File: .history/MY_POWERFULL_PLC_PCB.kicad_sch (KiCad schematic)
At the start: 6 parts, among them J1 DI_IN_Connector, J2 DI_IN_Connector, J3 DI_IN_Connector, J4 DI_IN_Connector, J5 DI_IN_Connector, J6 DI_IN_Connector

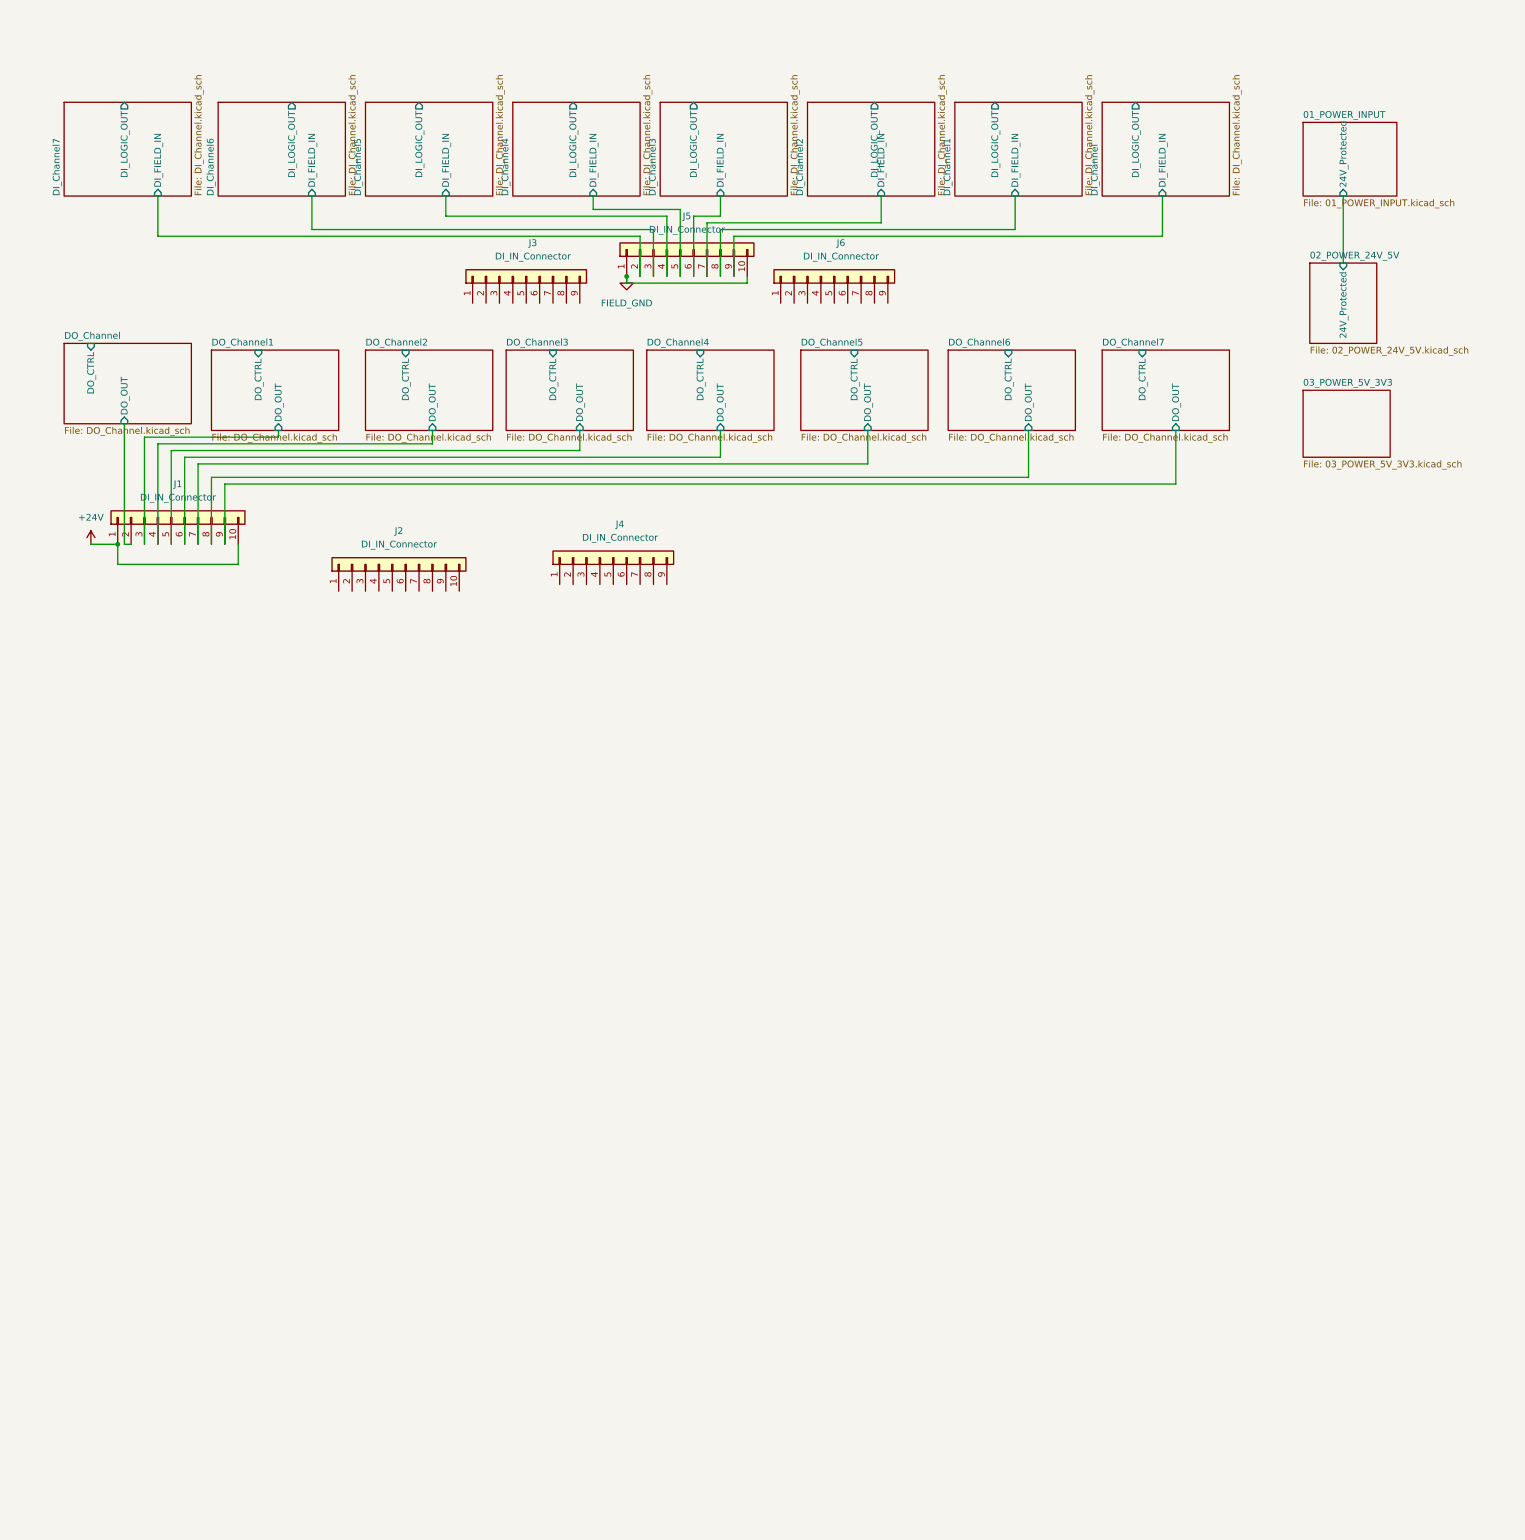
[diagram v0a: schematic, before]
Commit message: 112
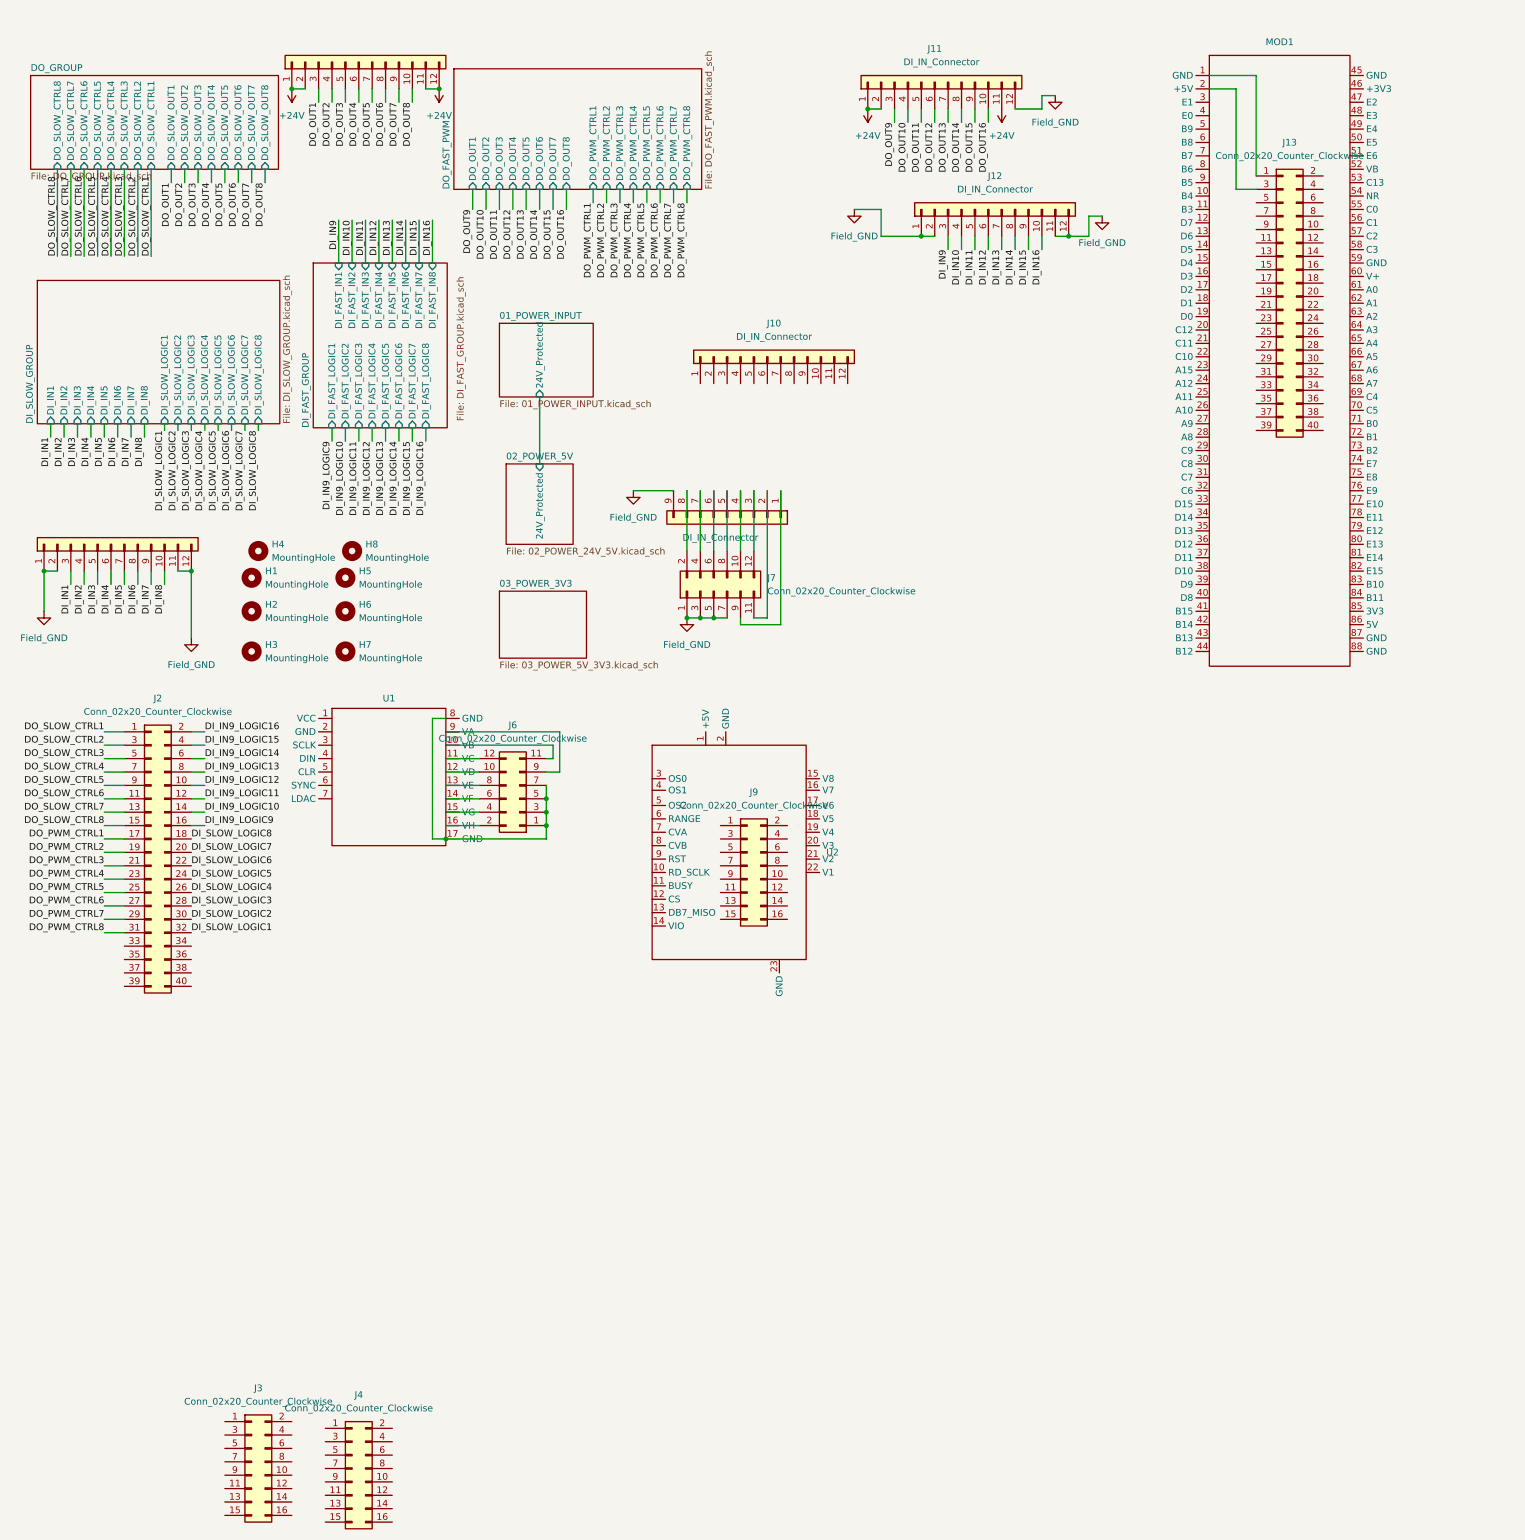
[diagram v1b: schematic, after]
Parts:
- removed J4: DI_IN_Connector, Connector_Phoenix_MC:PhoenixContact_MC_1,5_10-G-3.81_1x10_P3.81mm_Horizontal, symbol Connector_Generic:Conn_01x09
- added H1, H2, H3, H4, H5, H6, H7, H8: MountingHole, MountingHole:MountingHole_3.2mm_M3_Pad, symbol Mechanical:MountingHole
- added J13, J2: Conn_02x20_Counter_Clockwise, Connector_IDC:IDC-Header_2x20_P2.54mm_Vertical, symbol Connector_Generic:Conn_02x20_Odd_Even
- added J3, J4, J9: Conn_02x20_Counter_Clockwise, Connector_IDC:IDC-Header_2x08_P2.54mm_Vertical, symbol Connector_Generic:Conn_02x08_Odd_Even
- added J6, J7: Conn_02x20_Counter_Clockwise, Connector_IDC:IDC-Header_2x06_P2.54mm_Vertical, symbol Connector_Generic:Conn_02x06_Odd_Even
- added J8: DI_IN_Connector, Connector_Phoenix_MC:PhoenixContact_MC_1,5_9-G-3.5_1x09_P3.50mm_Horizontal, symbol Connector_Generic:Conn_01x09
- added MOD1: (no value), MyModules:WeAct_STM32H743VIT6, symbol MyModules:WeAct_STM32H743VIT6
- added U1: (no value), MyModules:DAC8568_Module_57x52mm, symbol MyModules:Module_DAC8568_8CH
- added U2: (no value), MyModules:AD7606_Module_40x30mm, symbol MyModules:Module_AD7606_8CH
- J1: renamed from J5; footprint Connector_Phoenix_MC:PhoenixContact_MC_1,5_10-G-3.81_1x10_P3.81mm_Horizontal -> Connector_Phoenix_MC:PhoenixContact_MC_1,5_12-G-3.5_1x12_P3.50mm_Horizontal; symbol Connector_Generic:Conn_01x10 -> Connector_Generic:Conn_01x12
- J10: renamed from J3; footprint Connector_Phoenix_MC:PhoenixContact_MC_1,5_10-G-3.81_1x10_P3.81mm_Horizontal -> Connector_Phoenix_MC:PhoenixContact_MC_1,5_12-G-3.5_1x12_P3.50mm_Horizontal; symbol Connector_Generic:Conn_01x09 -> Connector_Generic:Conn_01x12
- J11: renamed from J6; footprint Connector_Phoenix_MC:PhoenixContact_MC_1,5_10-G-3.81_1x10_P3.81mm_Horizontal -> Connector_Phoenix_MC:PhoenixContact_MC_1,5_12-G-3.5_1x12_P3.50mm_Horizontal; symbol Connector_Generic:Conn_01x09 -> Connector_Generic:Conn_01x12
- J12: renamed from J2; footprint Connector_Phoenix_MC:PhoenixContact_MC_1,5_10-G-3.81_1x10_P3.81mm_Horizontal -> Connector_Phoenix_MC:PhoenixContact_MC_1,5_12-G-3.5_1x12_P3.50mm_Horizontal; symbol Connector_Generic:Conn_01x10 -> Connector_Generic:Conn_01x12
- J5: renamed from J1; footprint Connector_Phoenix_MC:PhoenixContact_MC_1,5_10-G-3.81_1x10_P3.81mm_Horizontal -> Connector_Phoenix_MC:PhoenixContact_MC_1,5_12-G-3.5_1x12_P3.50mm_Horizontal; symbol Connector_Generic:Conn_01x10 -> Connector_Generic:Conn_01x12
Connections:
- net DI_Channel7/DI_FIELD_IN is gone; now on net Field_GND: J1.2 (Pin_2)
- net DO_Channel/DO_OUT is gone; now on net +24V: J5.2 (Pin_2)
- net +24V: now also J11.1 (Pin_1), J11.11 (Pin_11), J11.2 (Pin_2), J5.11 (Pin_11), J5.12 (Pin_12); no longer J5.10 (Pin_10)
- net DO_OUT9: now reaches J11.3 (Pin_3)
- net DO_OUT10: now reaches J11.4 (Pin_4)
- net DO_OUT11: now reaches J11.5 (Pin_5)
- net DO_OUT12: now reaches J11.6 (Pin_6)
- net DO_OUT13: now reaches J11.7 (Pin_7)
- net DO_OUT14: now reaches J11.8 (Pin_8)
- net DO_OUT15: now reaches J11.9 (Pin_9)
- net Field_GND: now reaches J12.1 (Pin_1)
- net Field_GND: now also J1.1 (Pin_1), J1.11 (Pin_11), J1.12 (Pin_12), J11.12 (Pin_12), J12.11 (Pin_11), J12.12 (Pin_12), J12.2 (Pin_2), J7.1 (Pin_1), J7.3 (Pin_3), J7.5 (Pin_5), J7.7 (Pin_7), J8.9 (Pin_9)
- net DI_IN16: now reaches J12.10 (Pin_10)
- net DI_IN9: now reaches J12.3 (Pin_3)
- net DI_IN10: now reaches J12.4 (Pin_4)
- net DI_IN11: now reaches J12.5 (Pin_5)
- net DI_IN12: now reaches J12.6 (Pin_6)
- net DI_IN13: now reaches J12.7 (Pin_7)
- net DI_IN14: now reaches J12.8 (Pin_8)
- net DI_IN15: now reaches J12.9 (Pin_9)
- net DI_Channel/DI_FIELD_IN renamed DI_IN7
- net DI_Channel1/DI_FIELD_IN renamed DI_IN6
- net DI_Channel2/DI_FIELD_IN renamed DI_IN5
- net DI_Channel3/DI_FIELD_IN renamed DI_IN4
- net DI_Channel4/DI_FIELD_IN renamed DI_IN3
- net DI_Channel5/DI_FIELD_IN renamed DI_IN2
- net DI_Channel6/DI_FIELD_IN renamed DI_IN1
- net DO_Channel1/DO_OUT renamed DO_OUT1
- net DO_Channel2/DO_OUT renamed DO_OUT2
- net DO_Channel3/DO_OUT renamed DO_OUT3
- net DO_Channel4/DO_OUT renamed DO_OUT4
- net DO_Channel5/DO_OUT renamed DO_OUT5
- net DO_Channel6/DO_OUT renamed DO_OUT6
- net DO_Channel7/DO_OUT renamed DO_OUT7
- net FIELD_GND renamed DI_IN8
- net DI_IN8: no longer J1.1 (Pin_1)
- new net: J13.1 (Pin_1), MOD1.1 (GND)
- new net: J13.3 (Pin_3), MOD1.2 (+5V)
- new net: J6.1 (Pin_1), J6.3 (Pin_3), J6.5 (Pin_5), J6.7 (Pin_7), U1.17 (GND), U1.8 (GND)
- new net: J6.10 (Pin_10), U1.12 (VD)
- new net: J6.11 (Pin_11), U1.10 (VB)
- new net: J6.12 (Pin_12), U1.11 (VC)
- new net: J6.2 (Pin_2), U1.16 (VH)
- new net: J6.4 (Pin_4), U1.15 (VG)
- new net: J6.6 (Pin_6), U1.14 (VF)
- new net: J6.8 (Pin_8), U1.13 (VE)
- new net: J6.9 (Pin_9), U1.9 (VA)
- new net: J7.10 (Pin_10), J8.4 (Pin_4)
- new net: J7.11 (Pin_11), J8.2 (Pin_2)
- new net: J7.12 (Pin_12), J8.3 (Pin_3)
- new net: J7.2 (Pin_2), J8.8 (Pin_8)
- new net: J7.4 (Pin_4), J8.7 (Pin_7)
- new net: J7.6 (Pin_6), J8.6 (Pin_6)
- new net: J7.8 (Pin_8), J8.5 (Pin_5)
- new net: J7.9 (Pin_9), J8.1 (Pin_1)
- new net DI_IN9_LOGIC10: J2.14 (Pin_14)
- new net DI_IN9_LOGIC11: J2.12 (Pin_12)
- new net DI_IN9_LOGIC12: J2.10 (Pin_10)
- new net DI_IN9_LOGIC13: J2.8 (Pin_8)
- new net DI_IN9_LOGIC14: J2.6 (Pin_6)
- new net DI_IN9_LOGIC15: J2.4 (Pin_4)
- new net DI_IN9_LOGIC16: J2.2 (Pin_2)
- new net DI_IN9_LOGIC9: J2.16 (Pin_16)
- new net DI_SLOW_LOGIC1: J2.32 (Pin_32)
- new net DI_SLOW_LOGIC2: J2.30 (Pin_30)
- new net DI_SLOW_LOGIC3: J2.28 (Pin_28)
- new net DI_SLOW_LOGIC4: J2.26 (Pin_26)
- new net DI_SLOW_LOGIC5: J2.24 (Pin_24)
- new net DI_SLOW_LOGIC6: J2.22 (Pin_22)
- new net DI_SLOW_LOGIC7: J2.20 (Pin_20)
- new net DI_SLOW_LOGIC8: J2.18 (Pin_18)
- new net DO_OUT16: J11.10 (Pin_10)
- new net DO_OUT8: J5.10 (Pin_10)
- new net DO_PWM_CTRL1: J2.17 (Pin_17)
- new net DO_PWM_CTRL2: J2.19 (Pin_19)
- new net DO_PWM_CTRL3: J2.21 (Pin_21)
- new net DO_PWM_CTRL4: J2.23 (Pin_23)
- new net DO_PWM_CTRL5: J2.25 (Pin_25)
- new net DO_PWM_CTRL6: J2.27 (Pin_27)
- new net DO_PWM_CTRL7: J2.29 (Pin_29)
- new net DO_PWM_CTRL8: J2.31 (Pin_31)
- new net DO_SLOW_CTRL1: J2.1 (Pin_1)
- new net DO_SLOW_CTRL2: J2.3 (Pin_3)
- new net DO_SLOW_CTRL3: J2.5 (Pin_5)
- new net DO_SLOW_CTRL4: J2.7 (Pin_7)
- new net DO_SLOW_CTRL5: J2.9 (Pin_9)
- new net DO_SLOW_CTRL6: J2.11 (Pin_11)
- new net DO_SLOW_CTRL7: J2.13 (Pin_13)
- new net DO_SLOW_CTRL8: J2.15 (Pin_15)
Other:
- sheet 02_POWER_24V_5V renamed 02_POWER_5V
- sheet 03_POWER_5V_3V3 renamed 03_POWER_3V3
- removed sheet DI_Channel
- removed sheet DI_Channel1
- removed sheet DI_Channel2
- removed sheet DI_Channel3
- removed sheet DI_Channel4
- removed sheet DI_Channel5
- removed sheet DI_Channel6
- removed sheet DI_Channel7
- removed sheet DO_Channel
- removed sheet DO_Channel1
- removed sheet DO_Channel2
- removed sheet DO_Channel3
- removed sheet DO_Channel4
- removed sheet DO_Channel5
- removed sheet DO_Channel6
- removed sheet DO_Channel7
- added sheet DI_FAST_GROUP (DI_FAST_GROUP.kicad_sch)
- added sheet DI_SLOW_GROUP (DI_SLOW_GROUP.kicad_sch)
- added sheet DO_FAST_PWM (DO_FAST_PWM.kicad_sch)
- added sheet DO_GROUP (DO_GROUP.kicad_sch)
